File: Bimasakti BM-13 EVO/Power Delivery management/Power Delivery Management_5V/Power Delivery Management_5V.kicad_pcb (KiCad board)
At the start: 4 copper layers, 42.4 x 42.4 mm, 24 parts, among them J1 +12V In, J2 Conn_01x03_Socket, J3 Slow Start

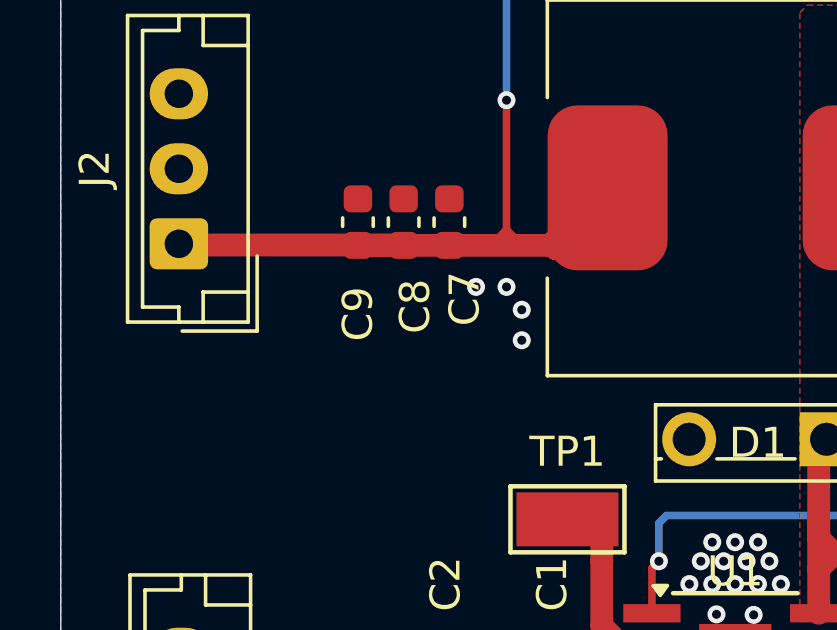
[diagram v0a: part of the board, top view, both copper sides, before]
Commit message: tambah led
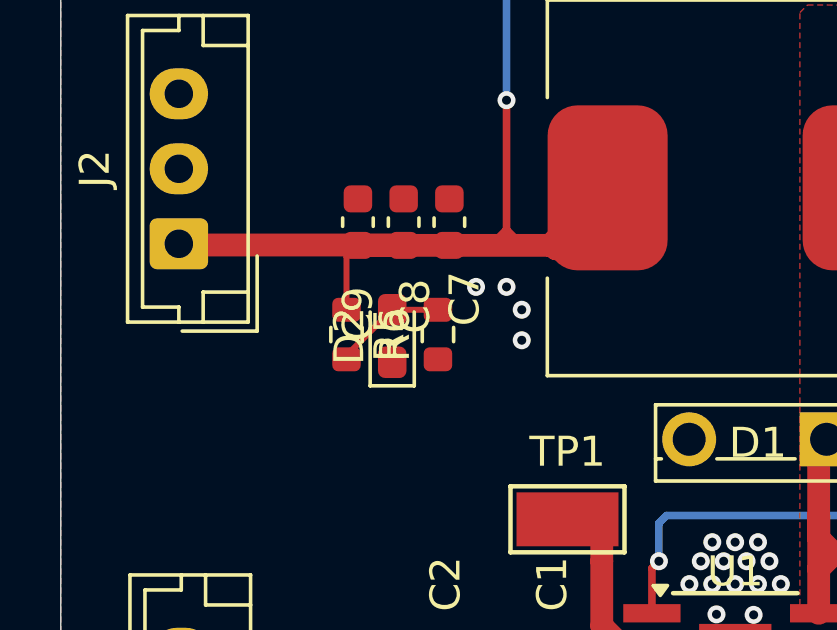
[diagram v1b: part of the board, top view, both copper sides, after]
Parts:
- added D2: LED, LED_SMD:LED_0603_1608Metric_Pad1.05x0.95mm_HandSolder, F.Cu at (64.3, 60.8)
- added R5: 1k, Resistor_SMD:R_0603_1608Metric, F.Cu at (62.7, 60.8)
- added R6: 1.5k, Resistor_SMD:R_0603_1608Metric, F.Cu at (65.8, 60.8)
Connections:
- net /+5V renamed +5v
- U1 pad 3: unconnected-(U1-EN-Pad3) -> EN
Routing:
- net Net-(D2-A): track 0.00 -> 3.81 mm
- net +5v: track 94.9 -> 97.2 mm
